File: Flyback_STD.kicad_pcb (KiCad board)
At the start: 2 copper layers, 59 x 30 mm, 46 parts, among them P1 BATT+, P2 BATT-, P3 VBUS, P4 GND, Q1 5N20A, T1 TRF-6, U1 OB2106MP, U2 VPC2188B, U4 TL431

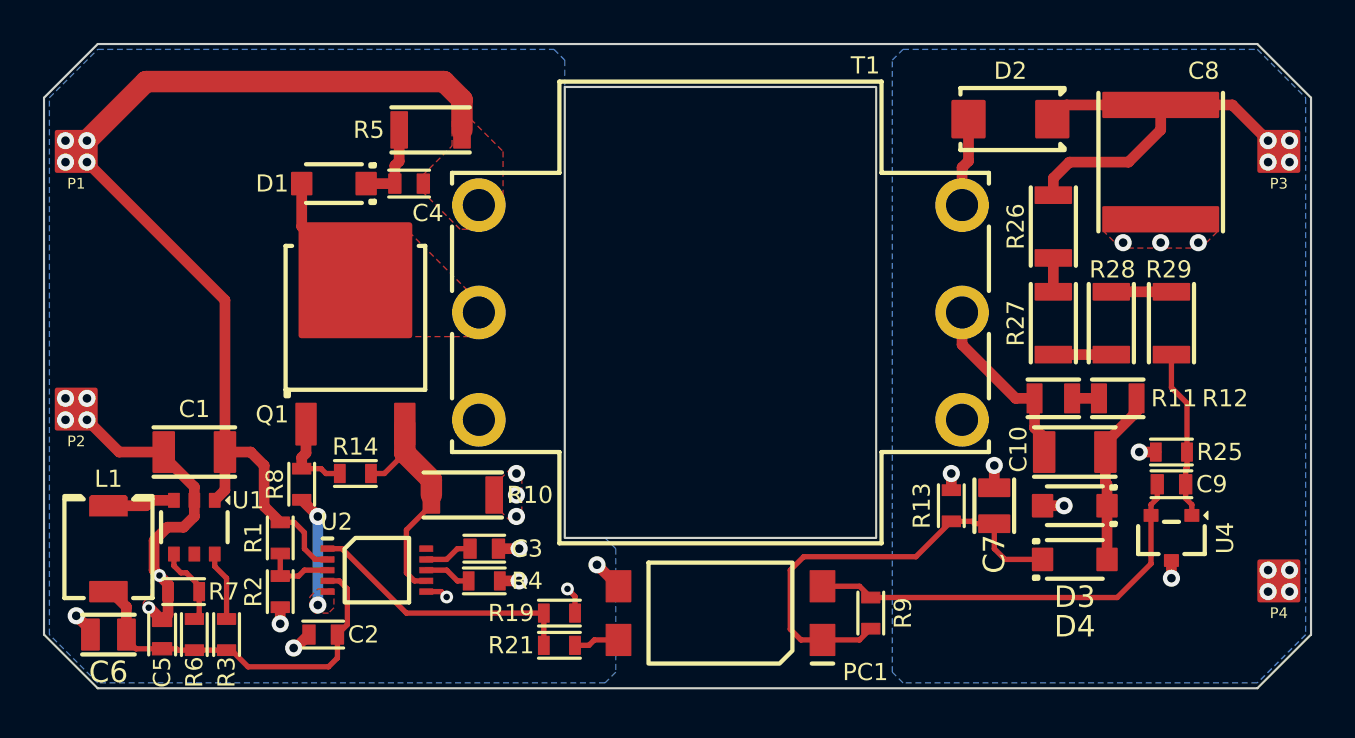
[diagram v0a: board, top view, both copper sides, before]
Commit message: Nightly update
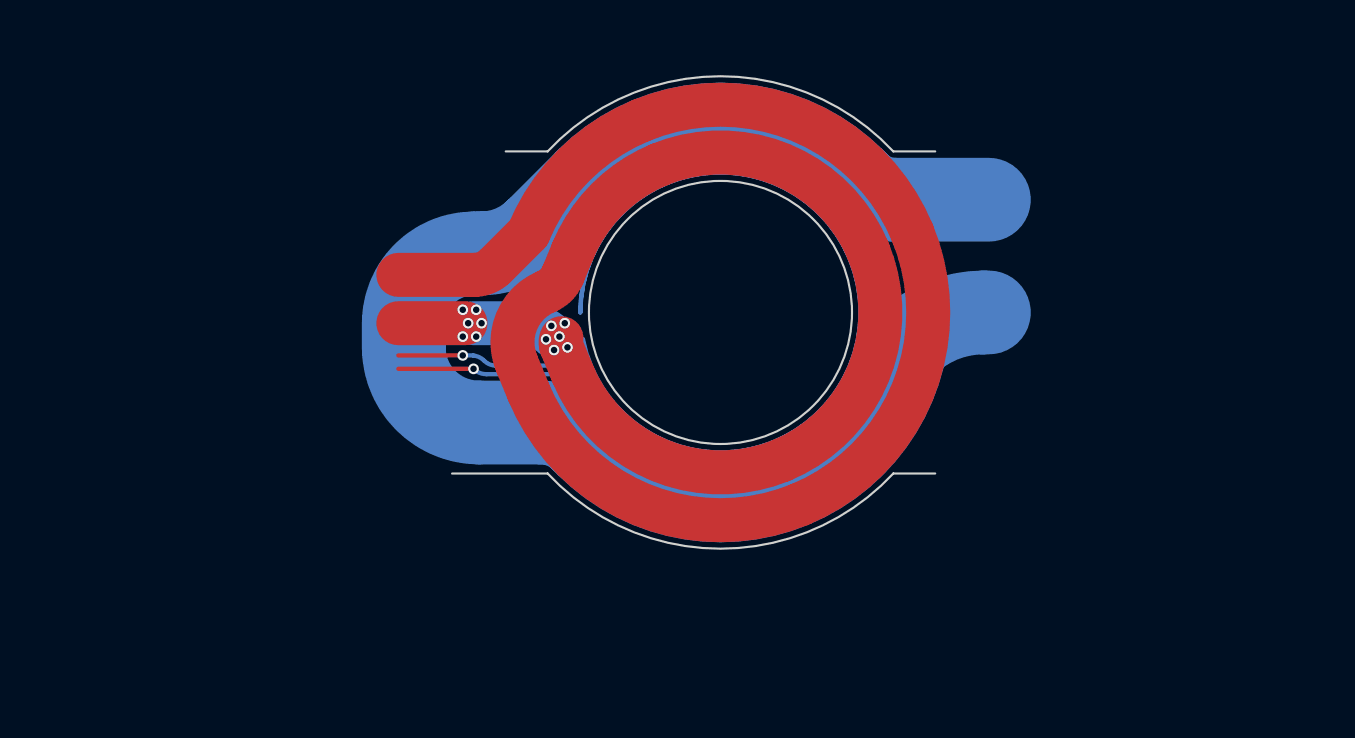
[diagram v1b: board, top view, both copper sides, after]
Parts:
- removed C1: 1uF, 001_GN_RCL_SMD:C1206(3216M)
- removed C10: 220pF, 001_GN_RCL_SMD:C1206(3216M)
- removed C2: 1uF, 001_GN_RCL_SMD:C0603(1608M)
- removed C3: 1nF, 001_GN_RCL_SMD:C0603(1608M)
- removed C4: 100pF, 001_GN_RCL_SMD:C0603(1608M)
- removed C5: 100nF, 001_GN_RCL_SMD:C0603(1608M)
- removed C6: 10uF, 001_GN_RCL_SMD:C0805(2012M)
- removed C7: 1uF, 001_GN_RCL_SMD:C0805(2012M)
- removed C8: 1uF, 001_GN_RCL_SMD:C2220(5650M)
- removed C9: 10nF, 001_GN_RCL_SMD:C0603(1608M)
- removed D1, D3, D4: DS110W, 002_GN_TWO-PIN_PLASTIC_SMD:SOD-123F
- removed D2: US1MF, 002_GN_TWO-PIN_PLASTIC_SMD:SMA(DO-214AC)
- removed L1: 100uH, 008_GN_POWER-CHOKE_SMD:MC-0420
- removed P1: BATT+, 302_MECH_PAD:SMP-Q_2020
- removed P2: BATT-, 302_MECH_PAD:SMP-Q_2020
- removed P3: VBUS, 302_MECH_PAD:SMP-Q_2020
- removed P4: GND, 302_MECH_PAD:SMP-Q_2020
- removed PC1: EL817S1(B)(TU)-F, MRLA:OC-4_6546
- removed Q1: 5N20A, 103_SP_POWER_TRANSISTOR_SMD:TO252-FET_6561
- removed R1: 100k, 001_GN_RCL_SMD:R0603(1608M)
- removed R10: 80mR/1W, 001_GN_RCL_SMD:R1206(3216M)
- removed R11, R12: 470k, 001_GN_RCL_SMD:R0805(2012M)
- removed R13: 2.2k, 001_GN_RCL_SMD:R0603(1608M)
- removed R14: 10k, 001_GN_RCL_SMD:R0603(1608M)
- removed R19: 5.6k, 001_GN_RCL_SMD:R0603(1608M)
- removed R2, R25, R7, R9: 4.7k, 001_GN_RCL_SMD:R0603(1608M)
- removed R21, R8: 22R, 001_GN_RCL_SMD:R0603(1608M)
- removed R26: 150k, 001_GN_RCL_SMD:R1206(3216M)
- removed R27, R28, R29: 200k, 001_GN_RCL_SMD:R1206(3216M)
- removed R3, R4: 22k, 001_GN_RCL_SMD:R0603(1608M)
- removed R5: 3.3k, 001_GN_RCL_SMD:R1206(3216M)
- removed R6: 20k, 001_GN_RCL_SMD:R0603(1608M)
- removed T1: TRF-6, MRLA:TRF-6_6P30S
- removed U1: OB2106MP, 003_GN_SMALL-SEMI_SMD:SOT-23-6
- removed U2: VPC2188B, 004_GN_MIDDLE-SEMI_SMD:MSOP-10_3030
- removed U4: TL431, 003_GN_SMALL-SEMI_SMD:SOT-23
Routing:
- net (no net): track 0.00 -> 241.5 mm, vias 0 -> 14
- net +BATT: track 48.8 -> 0.00 mm, vias 4 -> 0
- net GND: track 24.3 -> 0.00 mm, vias 17 -> 0
- net Net-(PC1-Pad1): track 21.0 -> 0.00 mm
- net Net-(C9-Pad1): track 20.0 -> 0.00 mm
- net VBUS: track 19.6 -> 0.00 mm, vias 4 -> 0
- net +10V: track 17.6 -> 0.00 mm
- net /COM: track 12.8 -> 0.00 mm
- net /CS: track 11.0 -> 0.00 mm
- net /SW_S2: track 8.60 -> 0.00 mm
- net Net-(C10-Pad2): track 8.13 -> 0.00 mm
- net /REF: track 7.93 -> 0.00 mm
- net /SW_P: track 5.54 -> 0.00 mm
- net /GT_U: track 5.21 -> 0.00 mm, vias 2 -> 0
- net GNDPWR: track 4.41 -> 0.00 mm, vias 12 -> 0
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- removed copper zone on F.Cu, net +BATT
- removed copper zone on F.Cu, net /GT_U
- removed copper zone on F.Cu, net /SW_P
- removed copper zone on B.Cu, net GND
- removed copper zone on F.Cu, net GND
- removed copper zone on B.Cu, net GNDPWR
- removed copper zone on F.Cu, net GNDPWR
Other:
- board size 59 x 30 mm -> 22.5 x 22 mm
- board text removed: "Flyback4MRLA_v0.9"
